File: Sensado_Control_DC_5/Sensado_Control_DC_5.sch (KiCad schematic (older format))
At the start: 92 parts, among them J1 Jumper, J2 Jumper, J3 Jumper, P1 R_FUENTE_CON, P10 GPIO, P2 I_+, P3 I_-, P4 POWER, P5 RS-232, P6 I2C, P7 SPI, P8 GND_REG, P9 RESET, Q1 NMOS, Q10 PMOS, Q11 NMOS, Q12 NMOS, Q13 NMOS, Q14 PMOS, Q15 PMOS, Q16 PMOS, Q2 NMOS, Q3 NMOS, Q4 NMOS, Q5 NMOS, Q6 PMOS, Q7 PMOS, Q8 PMOS, Q9 PMOS, U1 Atmega328PA, U2 ACS_712, U3 LD1117S50TR_FINAL, Y1 XRCHA_16M

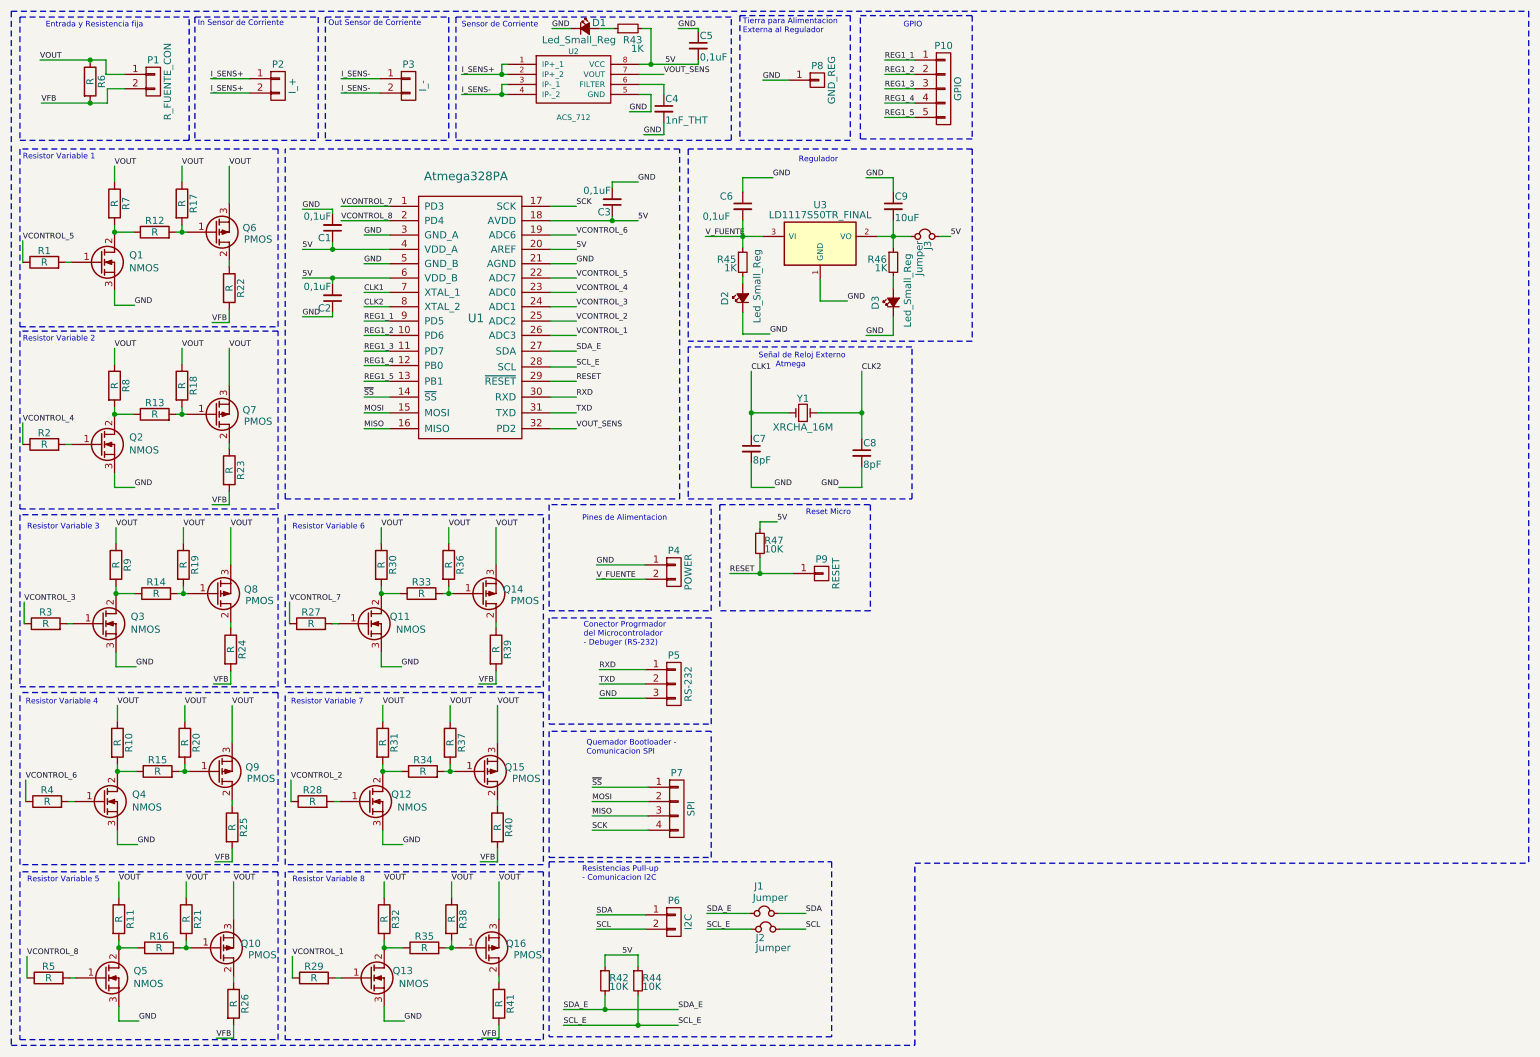
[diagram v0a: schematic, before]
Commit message: PCB mejorada
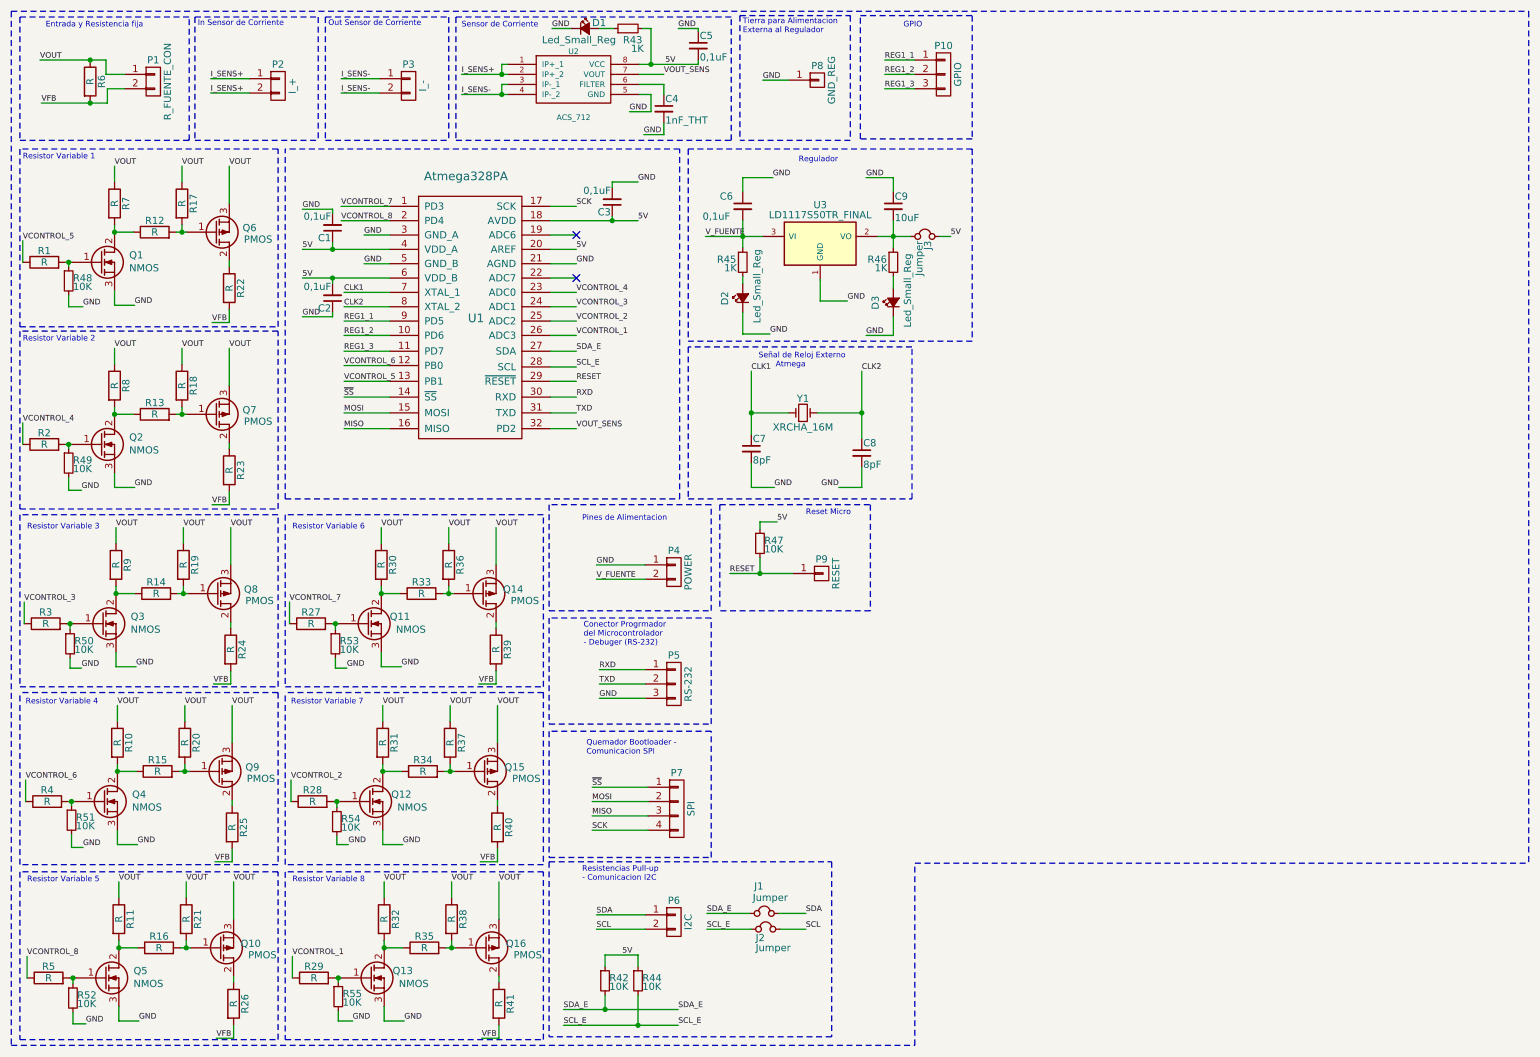
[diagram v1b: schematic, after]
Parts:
- removed P10: GPIO, Socket_Strips:Socket_Strip_Straight_1x05_Pitch2.54mm, symbol CONN_01X05
- added P10: GPIO, Socket_Strips:Socket_Strip_Straight_1x03_Pitch2.54mm, symbol CONN_01X03
- added R48, R49, R50, R51, R52, R53, R54, R55: 10K, Resistors_SMD:R_0805_HandSoldering, symbol 10K
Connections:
- net REG1_4 is gone; now on net VCONTROL_6: U1.12 (PB0)
- net REG1_5 is gone; now on net VCONTROL_5: U1.13 (PB1)
- net GND: now also R48.2, R49.2, R50.2, R51.2, R52.2, R53.2, R54.2, R55.2
- net REG1_1: now also P10.1 (P1)
- net REG1_2: now also P10.2 (P2)
- net REG1_3: now also P10.3 (P3)
- net VCONTROL_5: no longer U1.22 (ADC7)
- net VCONTROL_6: no longer U1.19 (ADC6)
- net at Q1.1 (G), R1.2: now also R48.1
- net at Q2.1 (G), R2.2: now also R49.1
- net at Q3.1 (G), R3.2: now also R50.1
- net at Q4.1 (G), R4.2: now also R51.1
- net at Q5.1 (G), R5.2: now also R52.1
- net at Q11.1 (G), R27.2: now also R53.1
- net at Q12.1 (G), R28.2: now also R54.1
- net at Q13.1 (G), R29.2: now also R55.1
- no-connect marks 0 -> 2

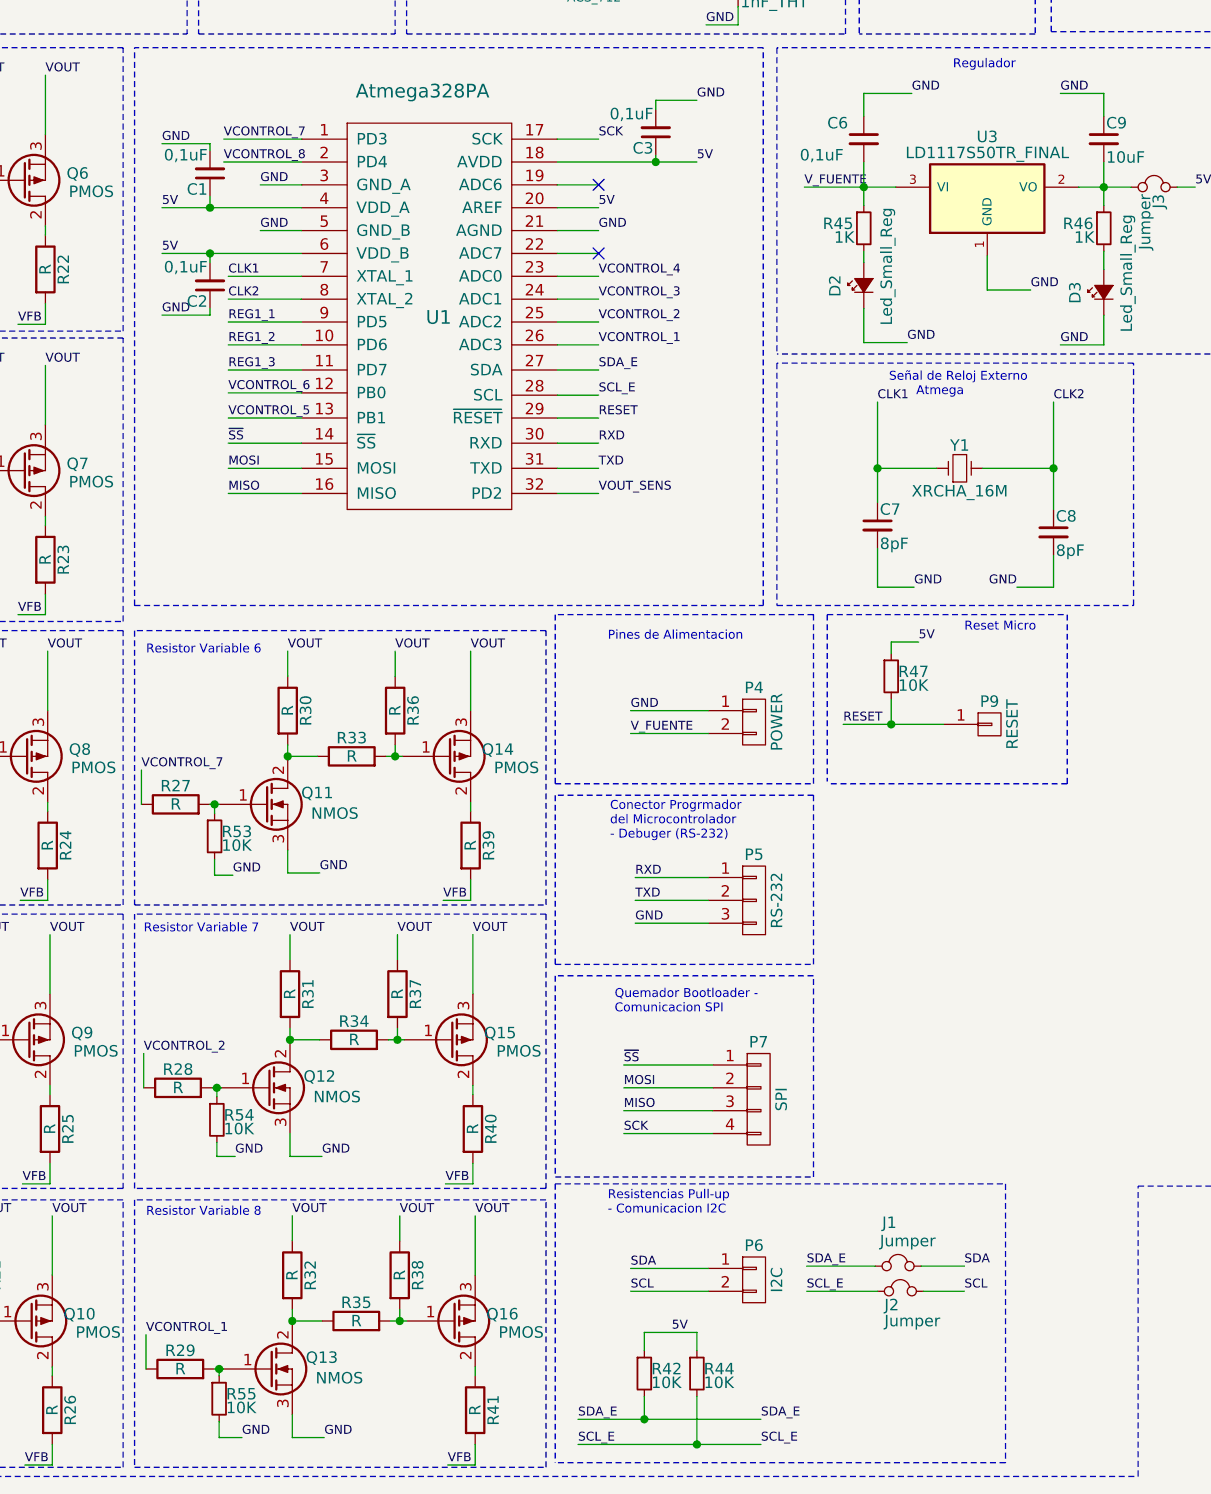
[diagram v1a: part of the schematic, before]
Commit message: Puertos I2C mejorados
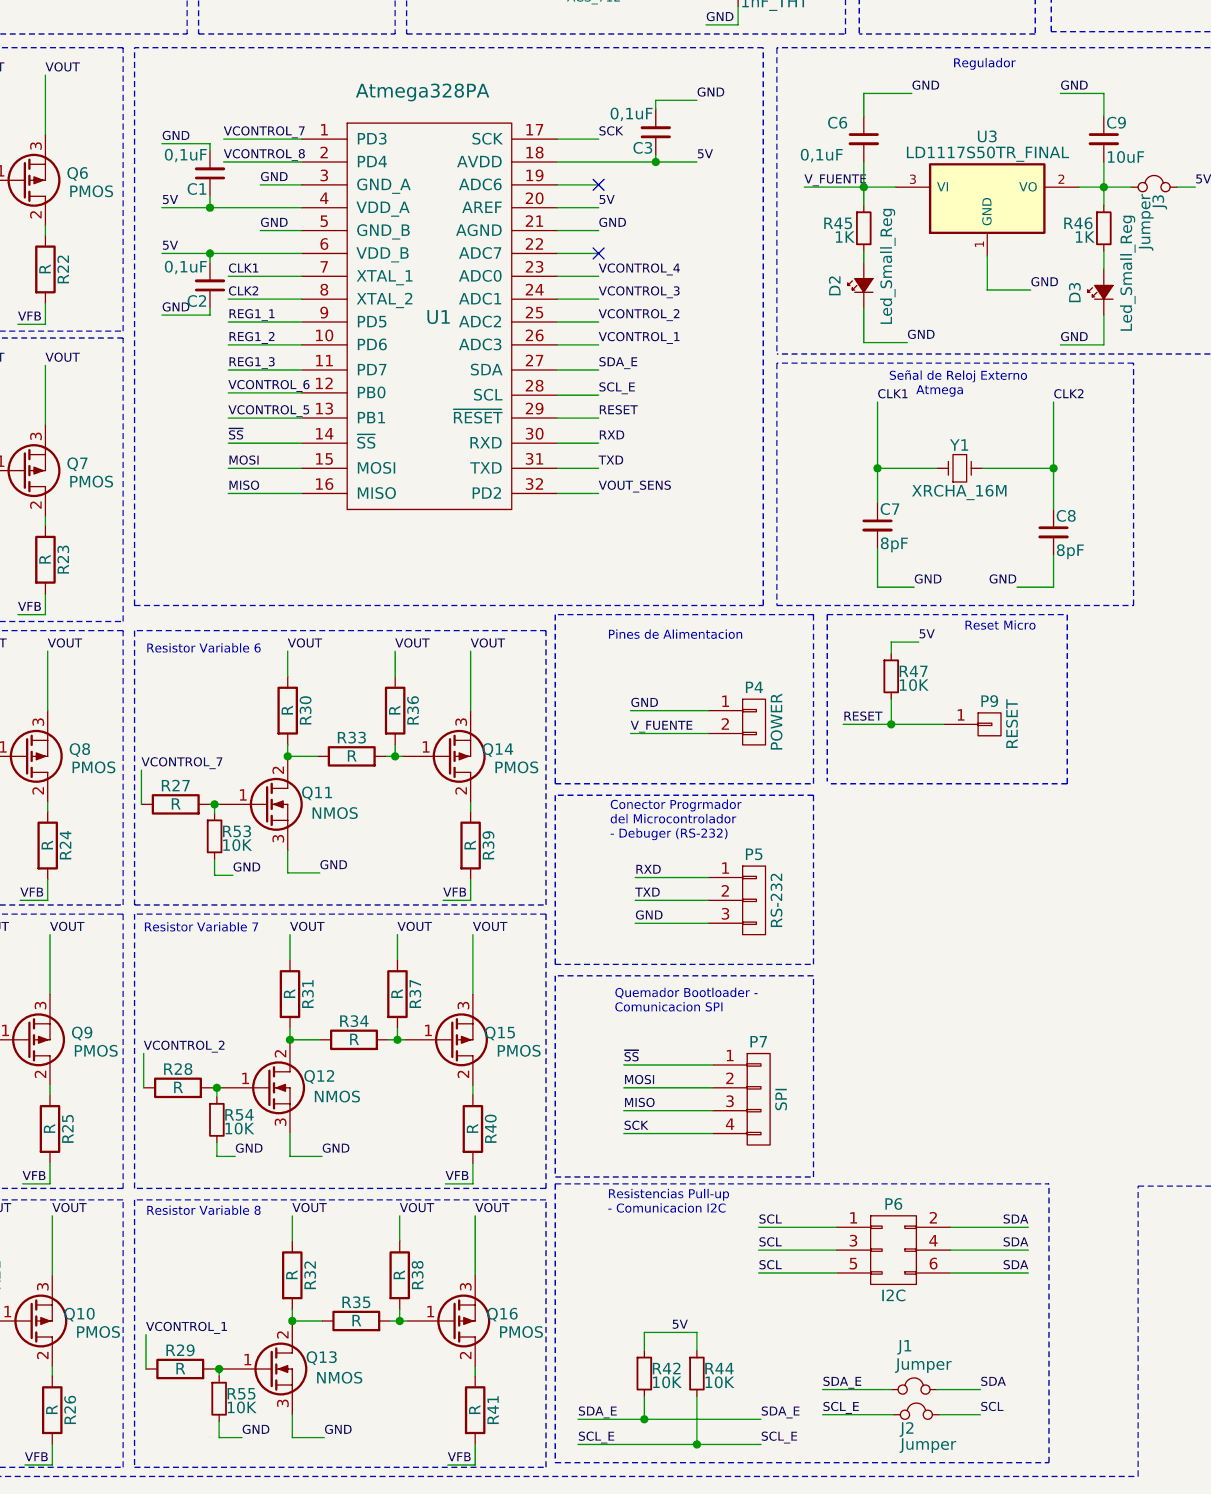
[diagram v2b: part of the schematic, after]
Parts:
- removed P6: I2C, Socket_Strips:Socket_Strip_Straight_1x02_Pitch2.54mm, symbol CONN_01X02
- added P6: I2C, Socket_Strips:Socket_Strip_Straight_2x03_Pitch2.54mm, symbol CONN_02X03
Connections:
- net SCL: now also P6.1 (P1), P6.3 (P3), P6.5 (P5)
- net SDA: now also P6.2 (P2), P6.4 (P4), P6.6 (P6)
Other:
- moved on the sheet: J1, J2
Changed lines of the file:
@@
 Text Label 4630 6250 0    39   ~ 0
 SCK
-$Comp
-L CONN_01X02 P6
-U 1 1 59DABC73
-P 5200 6890
-F 0 "P6" H 5200 7040 50  0000 C CNN
-F 1 "I2C" V 5300 6890 50  0000 C CNN
-F 2 "Socket_Strips:Socket_Strip_Straight_1x02_Pitch2.54mm" H 5200 6890 50  0001 C CNN
-F 3 "" H 5200 6890 50  0000 C CNN
-	1    5200 6890
-	1    0    0    -1
-$EndComp
-Text Label 4660 6840 0    39   ~ 0
+Text Label 6400 6760 2    39   ~ 0
 SDA
-Text Label 4660 6940 0    39   ~ 0
+Text Label 5220 6760 0    39   ~ 0
 SCL
 Text Notes 4560 6610 0    39   ~ 0
@@
 L Jumper J1
 U 1 1 59DB5A77
-P 5830 6830
-F 0 "J1" V 5640 6760 50  0000 L CNN
-F 1 "Jumper" V 5720 6750 50  0000 L CNN
-F 2 "Pin_Headers:Pin_Header_Straight_1x02_Pitch2.54mm" H 5830 6830 50  0001 C CNN
-F 3 "" H 5830 6830 50  0000 C CNN
-	1    5830 6830
+P 5900 7370
+F 0 "J1" V 5710 7300 50  0000 L CNN
+F 1 "Jumper" V 5790 7290 50  0000 L CNN
+F 2 "Pin_Headers:Pin_Header_Straight_1x02_Pitch2.54mm" H 5900 7370 50  0001 C CNN
+F 3 "" H 5900 7370 50  0000 C CNN
+	1    5900 7370
 	0    1    1    0
 $EndComp
@@
 L Jumper J2
 U 1 1 59DB5B56
-P 5840 6940
-F 0 "J2" V 5900 6870 50  0000 L CNN
-F 1 "Jumper" V 5970 6870 50  0000 L CNN
-F 2 "Pin_Headers:Pin_Header_Straight_1x02_Pitch2.54mm" H 5840 6940 50  0001 C CNN
-F 3 "" H 5840 6940 50  0000 C CNN
-	1    5840 6940
+P 5910 7480
+F 0 "J2" V 5970 7410 50  0000 L CNN
+F 1 "Jumper" V 6040 7410 50  0000 L CNN
+F 2 "Pin_Headers:Pin_Header_Straight_1x02_Pitch2.54mm" H 5910 7480 50  0001 C CNN
+F 3 "" H 5910 7480 50  0000 C CNN
+	1    5910 7480
 	0    1    1    0
 $EndComp
-Text Label 5430 6830 0    39   ~ 0
+Text Label 5500 7370 0    39   ~ 0
 SDA_E
-Text Label 5430 6940 0    39   ~ 0
+Text Label 5500 7480 0    39   ~ 0
 SCL_E
-Text Label 6120 6830 0    39   ~ 0
+Text Label 6190 7370 0    39   ~ 0
 SDA
-Text Label 6120 6940 0    39   ~ 0
+Text Label 6190 7480 0    39   ~ 0
 SCL
 Text Label 4350 660  0    39   ~ 0
@@
 	2490 3940 2490 1500
 Wire Wire Line
-	3220 2200 2610 2200
-Wire Wire Line
-	3220 2400 2610 2400
-Wire Wire Line
-	4950 2000 4340 2000
+	2610 2200 3220 2200
+Wire Wire Line
+	2610 2400 3220 2400
+Wire Wire Line
+	4340 2000 4950 2000
 Wire Wire Line
 	2880 1900 3220 1900
@@
 	5020 6250 4630 6250
 Wire Notes Line
-	4330 6470 6300 6470
-Wire Wire Line
-	5000 6840 4660 6840
-Wire Wire Line
-	5000 6940 4660 6940
+	4330 6470 6490 6470
+Wire Wire Line
+	6060 6760 6400 6760
+Wire Wire Line
+	5560 6760 5220 6760
 Wire Notes Line
 	4330 6470 4330 7690
@@
 Connection ~ 4950 7610
 Wire Wire Line
-	5430 6830 5730 6830
-Wire Wire Line
-	5430 6940 5740 6940
-Wire Wire Line
-	5930 6830 6120 6830
-Wire Wire Line
-	5940 6940 6120 6940
-Wire Notes Line
-	6300 6470 6300 7690
-Wire Notes Line
-	6300 7690 4330 7690
+	5500 7370 5800 7370
+Wire Wire Line
+	5500 7480 5810 7480
+Wire Wire Line
+	6000 7370 6190 7370
+Wire Wire Line
+	6010 7480 6190 7480
+Wire Notes Line
+	4330 7690 6490 7690
 Wire Wire Line
 	5040 660  5040 910
@@
 Wire Wire Line
 	2860 7580 2960 7580
+$Comp
+L CONN_02X03 P6
+U 1 1 59D41214
+P 5810 6760
+F 0 "P6" H 5810 6960 50  0000 C CNN
+F 1 "I2C" H 5810 6560 50  0000 C CNN
+F 2 "Socket_Strips:Socket_Strip_Straight_2x03_Pitch2.54mm" H 5810 5560 50  0001 C CNN
+F 3 "" H 5810 5560 50  0000 C CNN
+	1    5810 6760
+	1    0    0    -1
+$EndComp
+Text Label 5220 6660 0    39   ~ 0
+SCL
+Wire Wire Line
+	5560 6660 5220 6660
+Text Label 5220 6860 0    39   ~ 0
+SCL
+Wire Wire Line
+	5560 6860 5220 6860
+Text Label 6400 6660 2    39   ~ 0
+SDA
+Wire Wire Line
+	6060 6660 6400 6660
+Text Label 6400 6860 2    39   ~ 0
+SDA
+Wire Wire Line
+	6060 6860 6400 6860
+Wire Notes Line
+	6490 7690 6490 6470
 $EndSCHEMATC
